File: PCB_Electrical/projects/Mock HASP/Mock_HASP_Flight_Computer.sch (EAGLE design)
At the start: 10 parts

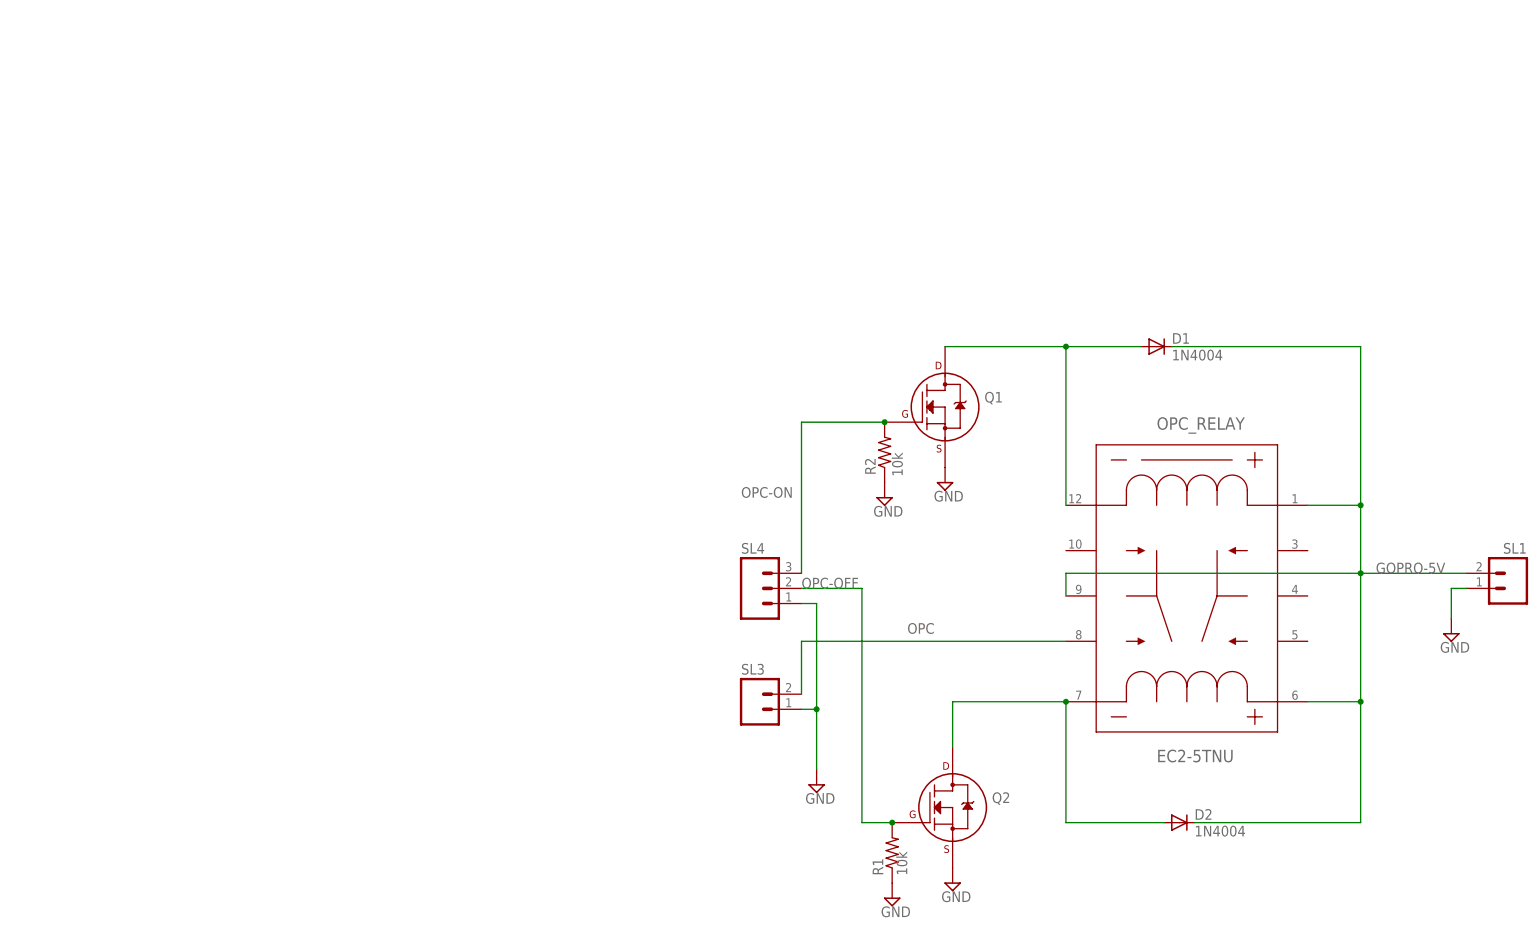
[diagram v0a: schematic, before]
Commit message: Added files for project schematics and boards that were developed this past summer
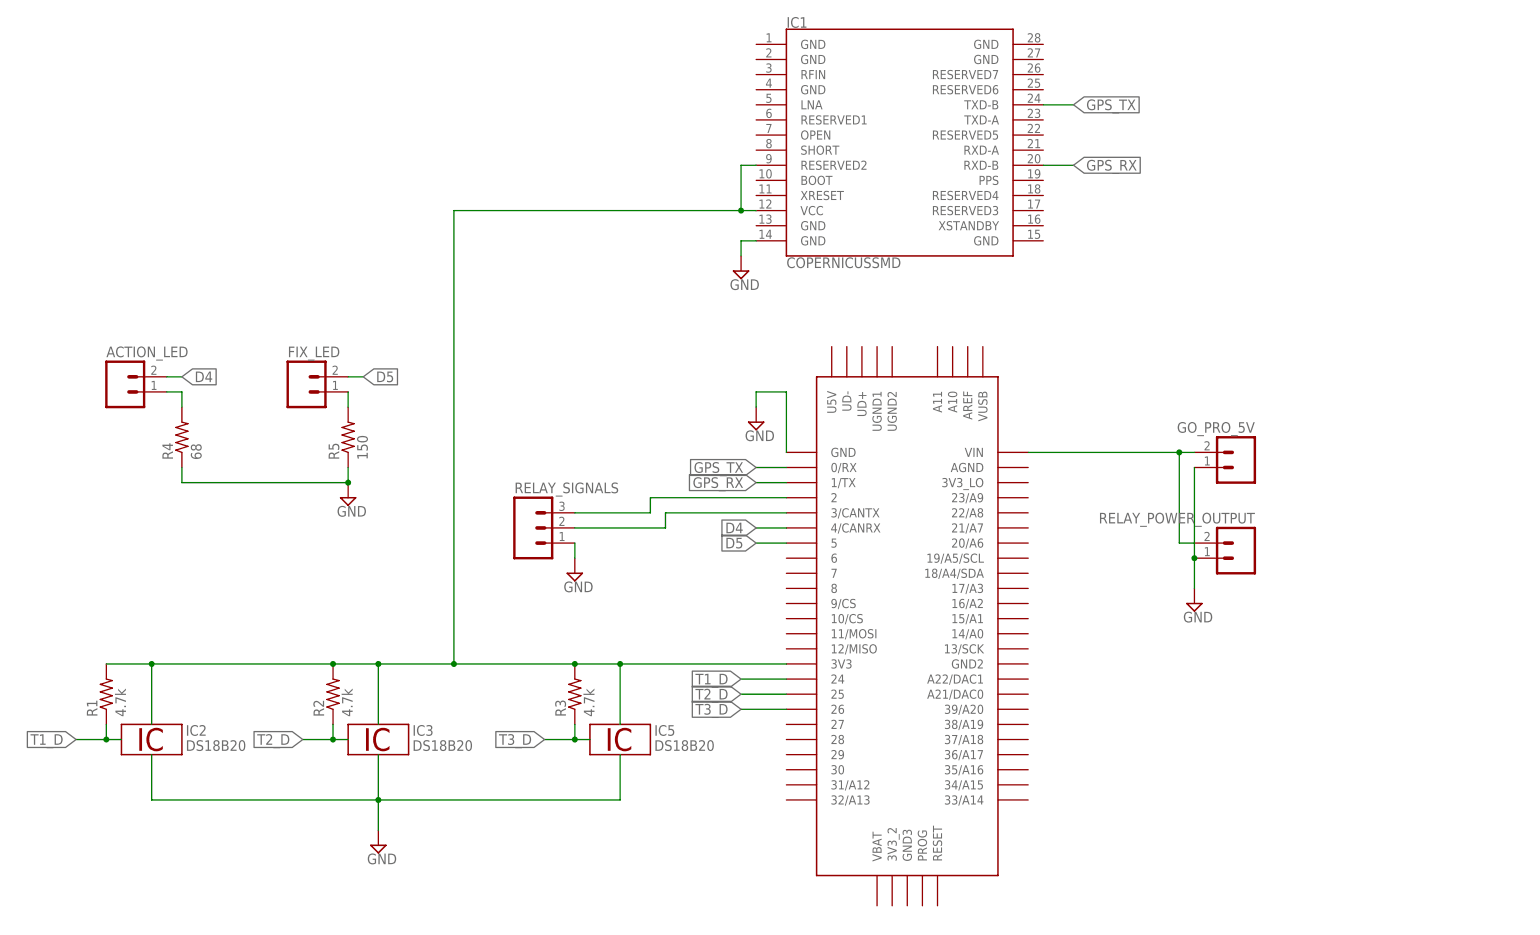
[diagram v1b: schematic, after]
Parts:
- removed D1, D2: 1N4004, diode:1N4004
- removed OPC_RELAY: EC2-5TNU, EC2-5TNU:EC2-5TNU
- removed Q1, Q2: (no value), transistors:2N7000_TO92
- removed SL1, SL3: (no value), con-amp-quick:M02
- removed SL4: (no value), con-amp-quick:M03
- added ACTION_LED, FIX_LED, GO_PRO_5V, RELAY_POWER_OUTPUT: (no value), con-amp-quick:M02
- added IC1: COPERNICUSSMD, SparkFun-GPS:COPERNICUSSMD
- added IC2, IC3, IC5: DS18B20, 1wire:DS18B20
- added R3: 4.7k, resistor:R-US_0207/10
- added R4: 68, resistor:R-US_0207/10
- added R5: 150, resistor:R-US_0207/10
- added RELAY_SIGNALS: (no value), con-amp-quick:M03
- added U$1: TEENSY_3.5/3.6, Teensy356:TEENSY_3.5/3.6
- R1, R2: value (none) -> 4.7k; device rcl:R-US_0207/7 -> resistor:R-US_0207/10
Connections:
- removed net GOPRO-5V: D1.C, D2.C, OPC_RELAY.1, OPC_RELAY.5, OPC_RELAY.8, SL1.2
- removed net OPC: OPC_RELAY.7, SL3.2
- removed net OPC-OFF: Q2.G, R1.2, SL4.2
- removed net OPC-ON: Q1.G, R2.2, SL4.3
- new net D4: ACTION_LED.2, U$1.4/CANRX
- new net D5: FIX_LED.2, U$1.5
- new net GPS_RX: IC1.RXD-B, U$1.1/TX
- new net GPS_TX: IC1.TXD-B, U$1.0/RX
- new net N$2: RELAY_SIGNALS.3, U$1.2
- new net N$4: ACTION_LED.1, R4.2
- new net N$5: GO_PRO_5V.2, RELAY_POWER_OUTPUT.2, U$1.VIN
- new net N$6: FIX_LED.1, R5.2
- new net T1_D: R1.1, U$1.24
- new net T2_D: R2.1, U$1.25
- new net T3_D: R3.1, U$1.26
- net GND: now also GO_PRO_5V.1, IC1.GND@5, R4.1, R5.1, RELAY_POWER_OUTPUT.1, RELAY_SIGNALS.1, U$1.GND; no longer Q1.S, Q2.S, R1.1, R2.1, SL1.1, SL3.1, SL4.1
- net N$1: now also IC1.RESERVED2, IC1.VCC, R1.2, R2.2, R3.2, U$1.3V3; no longer D1.A, OPC_RELAY.10, Q1.D
- net N$3: now also RELAY_SIGNALS.2, U$1.3/CANTX; no longer D2.A, OPC_RELAY.6, Q2.D
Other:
- note removed: "10k"
- moved on the sheet: R1, R2
